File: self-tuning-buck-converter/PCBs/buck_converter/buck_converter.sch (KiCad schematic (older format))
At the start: 52 parts, among them Q1 NMOS, U1 AMP from lab, U2 OPA2830, U3 LT1999-50, U4 LD1117V50, U6 ESP32-DEVKITC-32D, U7 IR2125, U8 MAX11644

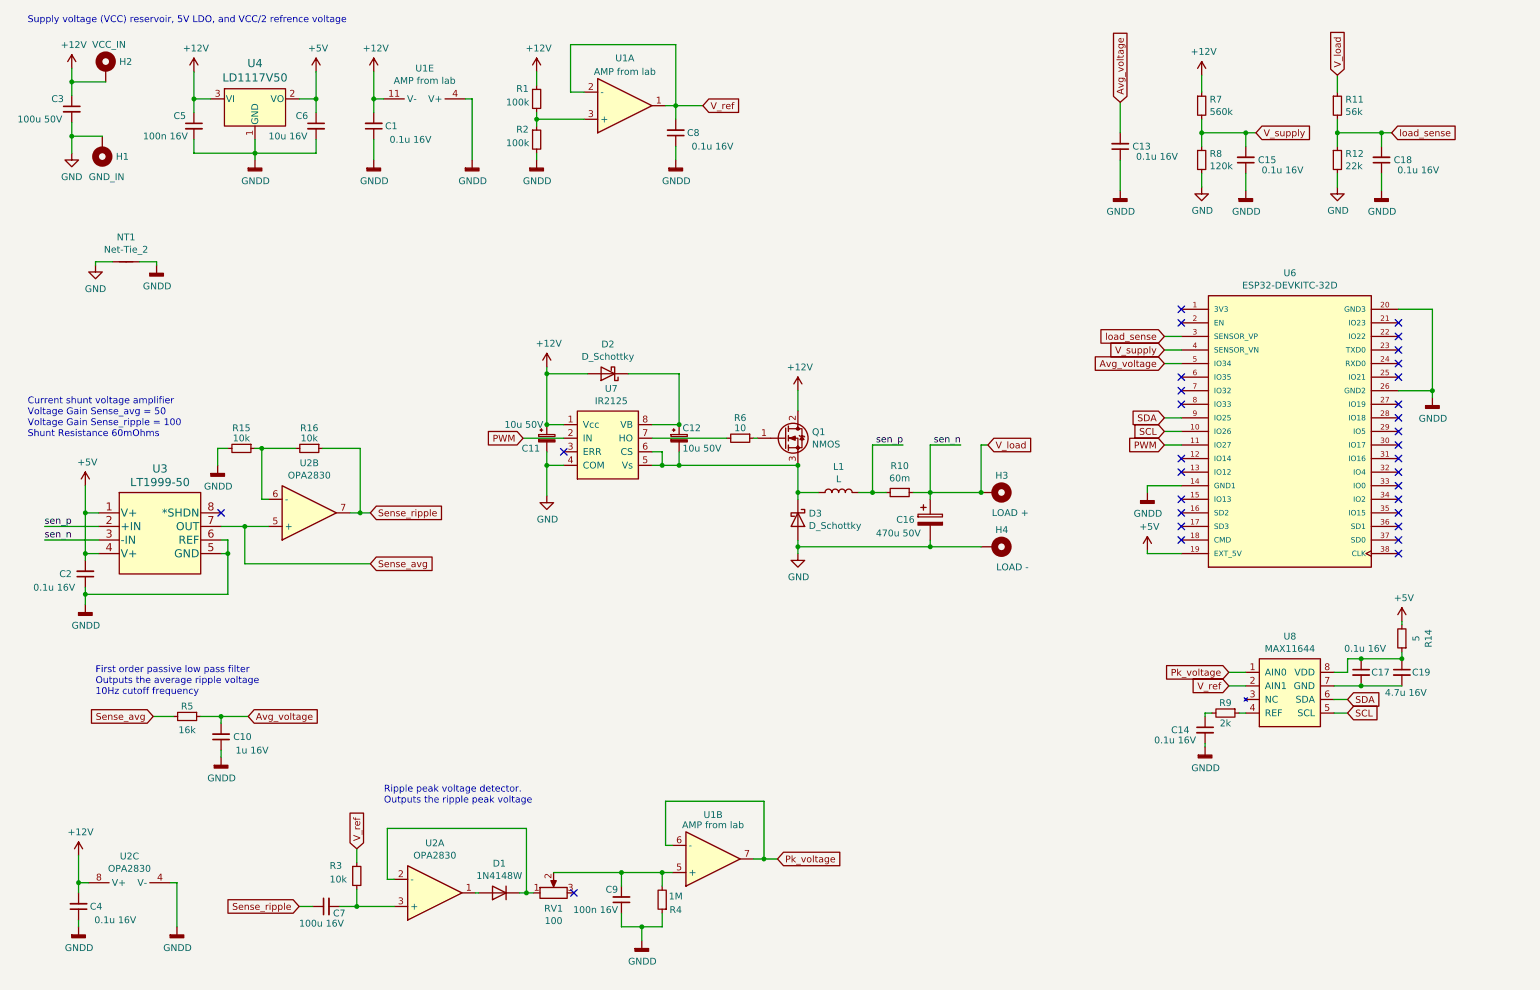
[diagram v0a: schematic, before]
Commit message: completed the PCB design
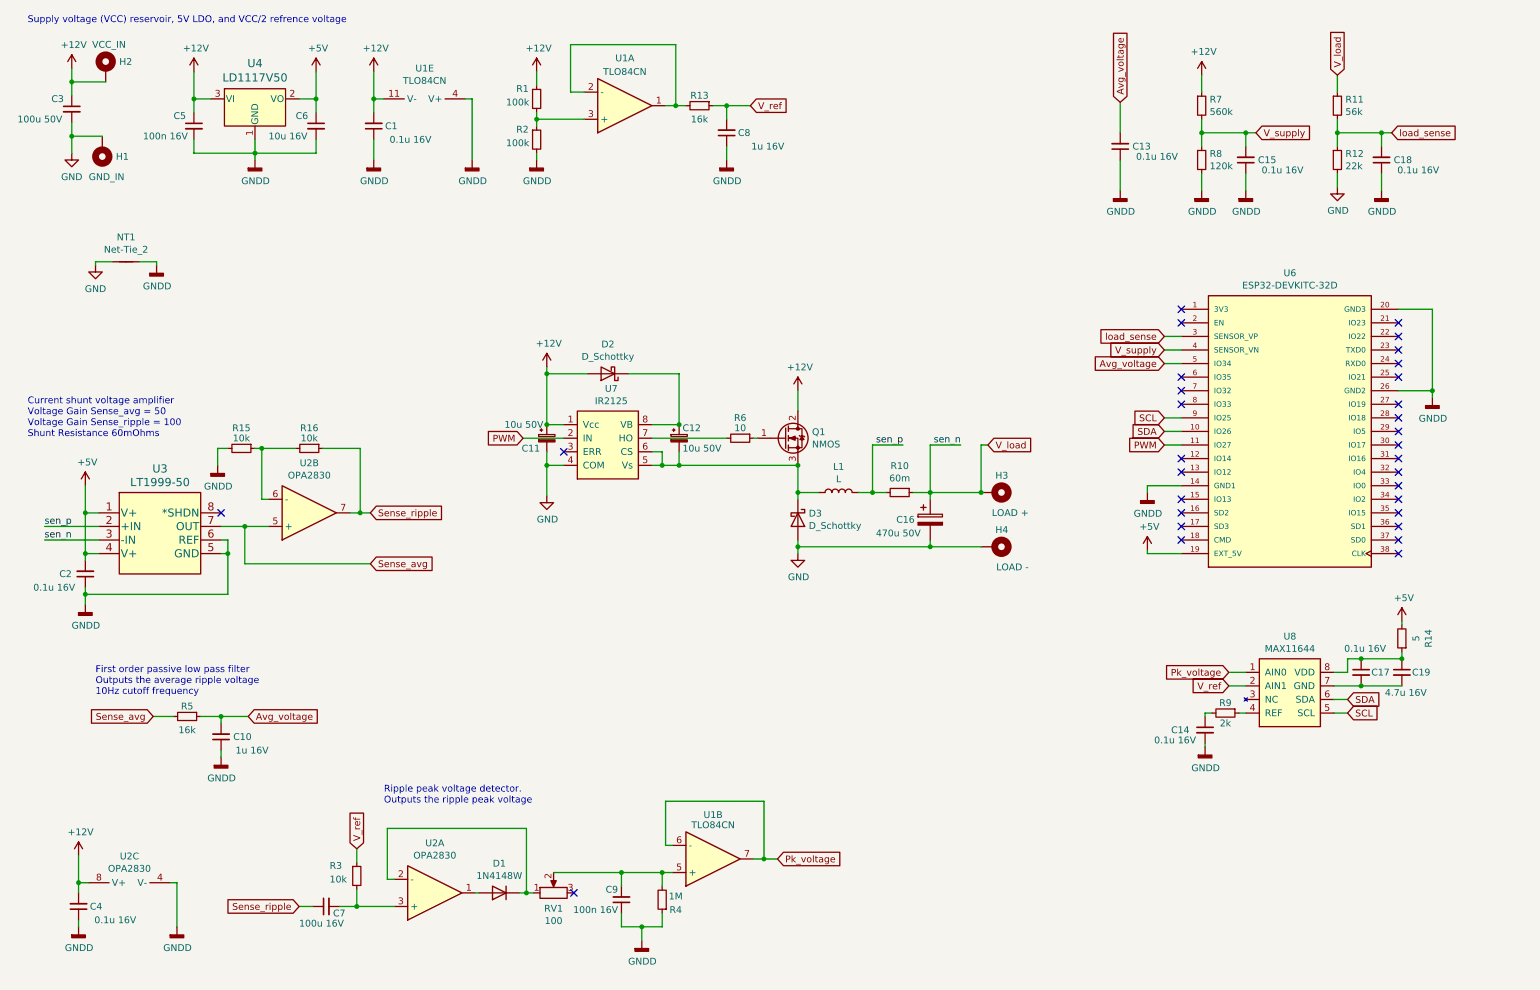
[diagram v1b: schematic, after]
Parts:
- added R13: 16k, Resistor_SMD:R_0603_1608Metric_Pad0.98x0.95mm_HandSolder, symbol Device:R_Small
- C8: value 0.1u 16V -> 1u 16V
- U1: value AMP from lab -> TLO84CN
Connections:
- net GND: no longer R8.2
- net GNDD: now also R8.2
- net SCL: now also U6.9 (IO25); no longer U6.10 (IO26)
- net SDA: now also U6.10 (IO26); no longer U6.9 (IO25)
- net V_ref: now also R13.1; no longer U1.1, U1.2 (-)
- new net: R13.2, U1.1, U1.2 (-)
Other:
- moved on the sheet: C8
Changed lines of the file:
@@
 	9250 1300 9250 1400
-$Comp
-L power:GND #PWR028
-U 1 1 6137E64C
-P 9250 1800
-F 0 "#PWR028" H 9250 1550 50  0001 C CNN
-F 1 "GND" H 9255 1627 50  0000 C CNN
-F 2 "" H 9250 1800 50  0001 C CNN
-F 3 "" H 9250 1800 50  0001 C CNN
-	1    9250 1800
-	1    0    0    -1
-$EndComp
 $Comp
 L power:+12V #PWR027
@@
 Wire Wire Line
 	10250 1400 10250 1500
-Wire Wire Line
-	9250 1700 9250 1800
 $Comp
 L power:GNDD #PWR030
@@
 P 3525 1250
 F 0 "U1" V 3200 1250 50  0000 C CNN
-F 1 "AMP from lab" V 3291 1250 50  0000 C CNN
+F 1 "TLO84CN" V 3291 1250 50  0000 C CNN
 F 2 "Package_DIP:DIP-14_W7.62mm" H 3525 1250 50  0001 C CNN
 F 3 "~" H 3525 1250 50  0001 C CNN
@@
 Wire Wire Line
 	8975 3500 9100 3500
+Text GLabel 8975 3500 0    50   Input ~ 0
+SCL
 Text GLabel 8975 3600 0    50   Input ~ 0
-SCL
-Text GLabel 8975 3500 0    50   Input ~ 0
 SDA
 Wire Wire Line
@@
 P 5000 1200
 F 0 "U1" H 5000 850 50  0000 C CNN
-F 1 "AMP from lab" H 5000 950 50  0000 C CNN
+F 1 "TLO84CN" H 5000 950 50  0000 C CNN
 F 2 "Package_DIP:DIP-14_W7.62mm" H 5000 1200 50  0001 C CNN
 F 3 "~" H 5000 1200 50  0001 C CNN
@@
 $EndComp
 Wire Wire Line
-	5375 1500 5375 1600
-Wire Wire Line
-	5375 1200 5375 1300
+	5750 1500 5750 1600
+Wire Wire Line
+	5750 1200 5750 1300
 $Comp
 L power:GNDD #PWR016
 U 1 1 6193F07B
-P 5375 1600
-F 0 "#PWR016" H 5375 1350 50  0001 C CNN
-F 1 "GNDD" H 5379 1445 50  0000 C CNN
-F 2 "" H 5375 1600 50  0001 C CNN
-F 3 "" H 5375 1600 50  0001 C CNN
-	1    5375 1600
+P 5750 1600
+F 0 "#PWR016" H 5750 1350 50  0001 C CNN
+F 1 "GNDD" H 5754 1445 50  0000 C CNN
+F 2 "" H 5750 1600 50  0001 C CNN
+F 3 "" H 5750 1600 50  0001 C CNN
+	1    5750 1600
 	1    0    0    -1
 $EndComp
@@
 L Device:C_Small C8
 U 1 1 61934821
-P 5375 1400
-F 0 "C8" H 5550 1400 50  0000 R CNN
-F 1 "0.1u 16V" H 5800 1500 50  0000 R CNN
-F 2 "Capacitor_SMD:C_0603_1608Metric_Pad1.08x0.95mm_HandSolder" H 5375 1400 50  0001 C CNN
-F 3 "~" H 5375 1400 50  0001 C CNN
-	1    5375 1400
+P 5750 1400
+F 0 "C8" H 5925 1400 50  0000 R CNN
+F 1 "1u 16V" H 6175 1500 50  0000 R CNN
+F 2 "Capacitor_SMD:C_0603_1608Metric_Pad1.08x0.95mm_HandSolder" H 5750 1400 50  0001 C CNN
+F 3 "~" H 5750 1400 50  0001 C CNN
+	1    5750 1400
 	1    0    0    1
 $EndComp
-Text GLabel 5575 1200 2    50   Input ~ 0
+Text GLabel 5925 1200 2    50   Input ~ 0
 V_ref
-Connection ~ 5375 1200
-Wire Wire Line
-	5375 1200 5575 1200
 Wire Wire Line
 	4350 1300 4350 1350
@@
 P 5650 6750
 F 0 "U1" H 5650 6425 50  0000 C CNN
-F 1 "AMP from lab" H 5650 6500 50  0000 C CNN
+F 1 "TLO84CN" H 5650 6500 50  0000 C CNN
 F 2 "Package_DIP:DIP-14_W7.62mm" H 5650 6750 50  0001 C CNN
 F 3 "~" H 5650 6750 50  0001 C CNN
@@
 Wire Wire Line
 	1550 2350 1550 2375
+$Comp
+L Device:R_Small R13
+U 1 1 6160E070
+P 5550 1200
+F 0 "R13" V 5475 1200 50  0000 C CNN
+F 1 "16k" V 5650 1200 50  0000 C CNN
+F 2 "Resistor_SMD:R_0603_1608Metric_Pad0.98x0.95mm_HandSolder" H 5550 1200 50  0001 C CNN
+F 3 "~" H 5550 1200 50  0001 C CNN
+F 4 "RR0816P-163-D" V 5550 1200 50  0001 C CNN "Part Number"
+	1    5550 1200
+	0    1    1    0
+$EndComp
+Wire Wire Line
+	5375 1200 5450 1200
+Connection ~ 5375 1200
+Wire Wire Line
+	5650 1200 5750 1200
+Wire Wire Line
+	5750 1200 5925 1200
+Connection ~ 5750 1200
+$Comp
+L power:GNDD #PWR?
+U 1 1 616B9AA7
+P 9250 1825
+F 0 "#PWR?" H 9250 1575 50  0001 C CNN
+F 1 "GNDD" H 9254 1670 50  0000 C CNN
+F 2 "" H 9250 1825 50  0001 C CNN
+F 3 "" H 9250 1825 50  0001 C CNN
+	1    9250 1825
+	1    0    0    -1
+$EndComp
+Wire Wire Line
+	9250 1700 9250 1825
 $EndSCHEMATC

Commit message: many images added for the final report... also tidied up the schematic for input into the report
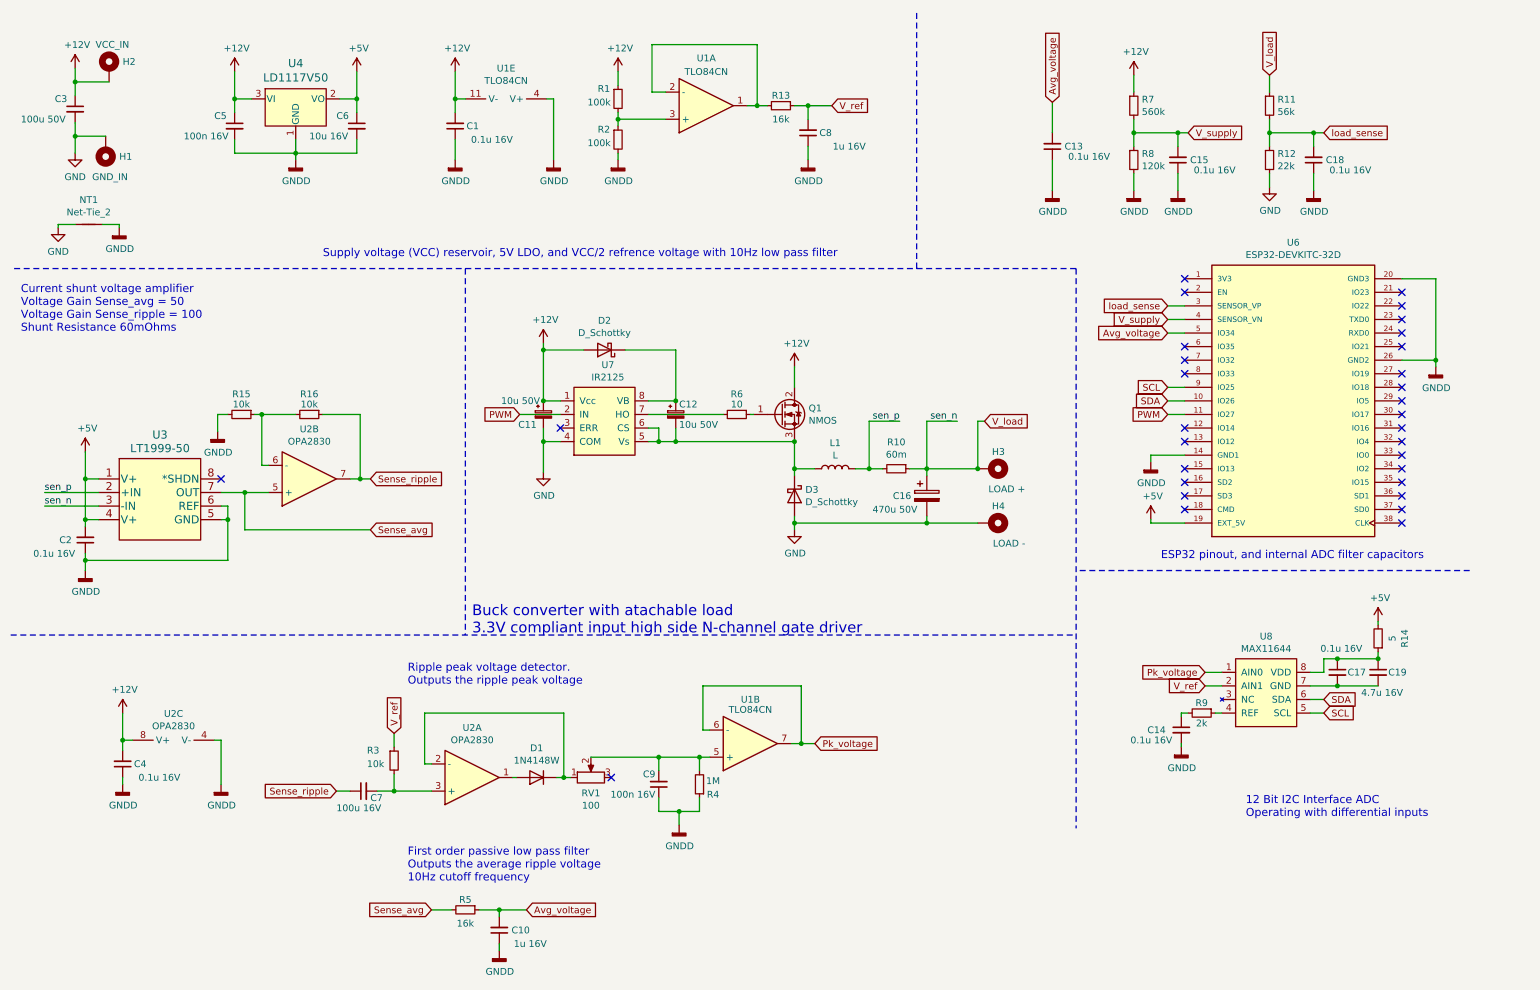
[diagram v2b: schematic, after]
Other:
- note added: "12 Bit I2C Interface ADC\nOperating with differential inputs"
- note added: "Buck converter with atachable load\n3.3V compliant input high side N-channel gate driver\n"
- note added: "ESP32 pinout, and internal ADC filter capacitors"
- note added: "Supply voltage (VCC) reservoir, 5V LDO, and VCC/2 refrence voltage with 10Hz low pass filter\n"
- note removed: "Supply voltage (VCC) reservoir, 5V LDO, and VCC/2 refrence voltage"
- moved on the sheet: C1, C10, C11, C12, C13, C14, C15, C16, C17, C18, C19, C2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
